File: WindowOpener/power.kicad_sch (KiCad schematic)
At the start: 18 parts, among them J10 Batt_Conn1, J11 Batt_Conn2, J12 Batt_Conn2, J3 Batt_Conn1, J4 Batt_Conn2, J5 Batt_Conn1, J6 Batt_Conn2, J7 Batt_Conn1, J8 Batt_Conn2, J9 Batt_Conn2, U3 AZ1117CH2-3.3, U4 PAM2421AECADJR

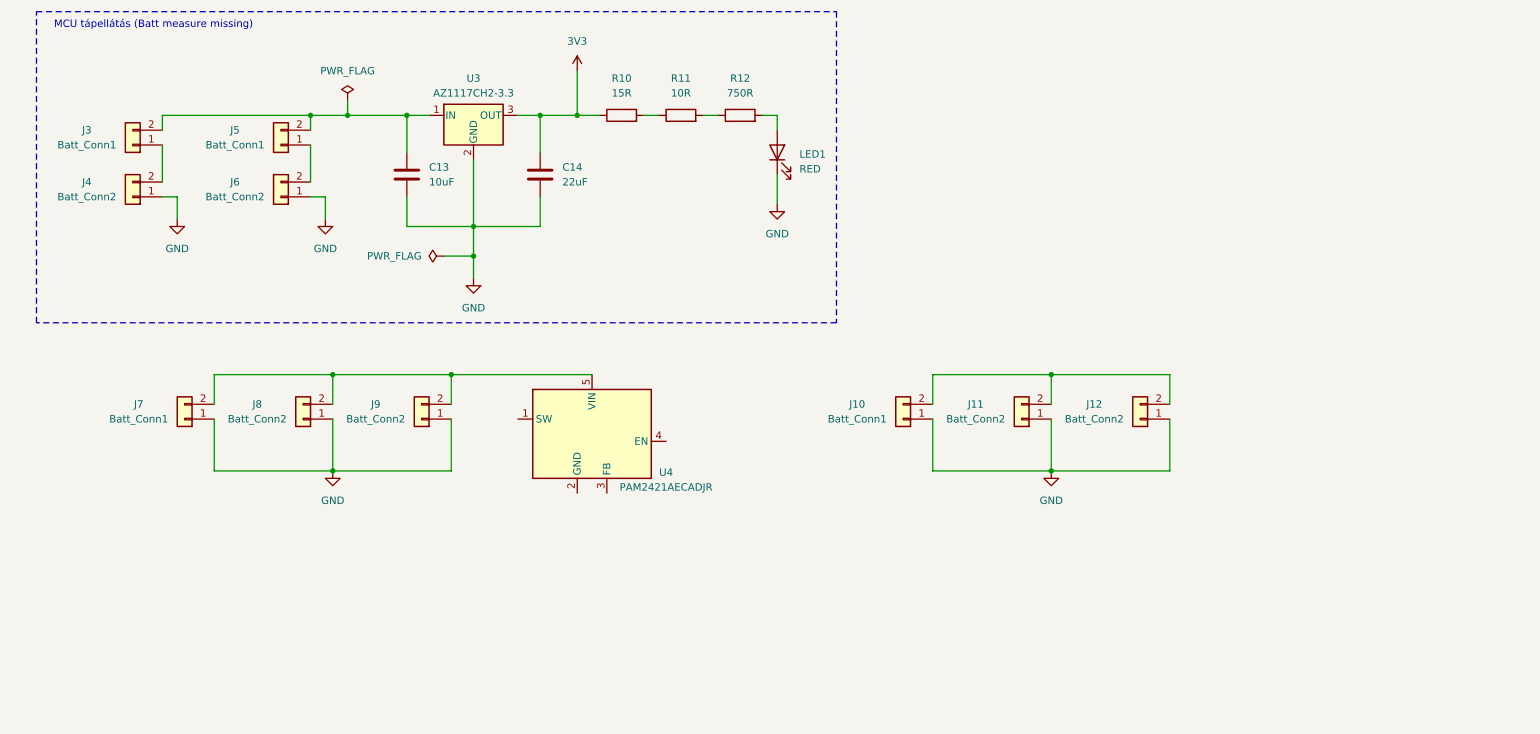
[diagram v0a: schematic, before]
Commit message: v0.2
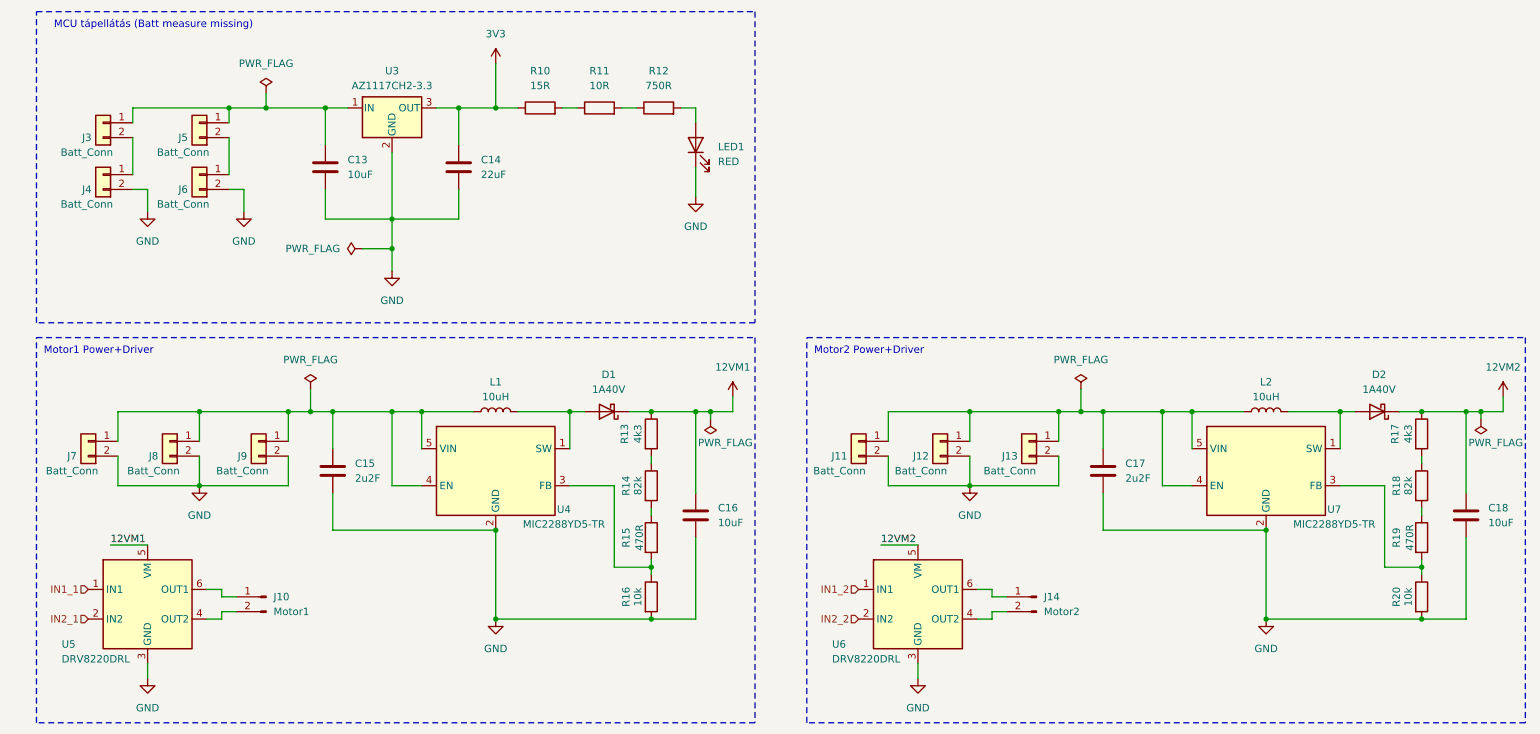
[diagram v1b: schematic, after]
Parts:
- removed J10: Batt_Conn1, Battery:BatteryHolder_Keystone_1042_1x18650, symbol Connector_Generic:Conn_01x02
- added C15, C17: 2u2F, Capacitor_SMD:C_1206_3216Metric_Pad1.33x1.80mm_HandSolder, symbol Device:C
- added C16, C18: 10uF, Capacitor_SMD:C_1206_3216Metric_Pad1.33x1.80mm_HandSolder, symbol Device:C
- added D1, D2: 1A40V, SmartHomeFootprints:1N5819HW-7-F, symbol Device:D_Schottky
- added J10: Motor1, Connector_PinHeader_2.54mm:PinHeader_1x02_P2.54mm_Vertical, symbol Connector:Conn_01x02_Pin
- added J13: Batt_Conn, Battery:BatteryHolder_Keystone_1042_1x18650, symbol Connector_Generic:Conn_01x02
- added J14: Motor2, Connector_PinHeader_2.54mm:PinHeader_1x02_P2.54mm_Vertical, symbol Connector:Conn_01x02_Pin
- added L1, L2: 10uH, Inductor_SMD:L_1210_3225Metric_Pad1.42x2.65mm_HandSolder, symbol Device:L
- added R13, R17: 4k3, Resistor_SMD:R_1206_3216Metric_Pad1.30x1.75mm_HandSolder, symbol Device:R
- added R14, R18: 82k, Resistor_SMD:R_1206_3216Metric_Pad1.30x1.75mm_HandSolder, symbol Device:R
- added R15, R19: 470R, Resistor_SMD:R_1206_3216Metric_Pad1.30x1.75mm_HandSolder, symbol Device:R
- added R16, R20: 10k, Resistor_SMD:R_2010_5025Metric_Pad1.40x2.65mm_HandSolder, symbol Device:R
- added U5, U6: DRV8220DRL, Package_TO_SOT_SMD:SOT-563, symbol Driver_Motor:DRV8220DRL
- added U7: MIC2288YD5-TR, Package_TO_SOT_SMD:TSOT-23-5_HandSoldering, symbol SmartHomeSymbols:PAM2421AECADJR
- C13: footprint Capacitor_SMD:C_2220_5750Metric_Pad1.97x5.40mm_HandSolder -> Capacitor_SMD:C_1206_3216Metric_Pad1.33x1.80mm_HandSolder; Store link https://hu.farnell.com/chemi-con/kts500b106m55n0t00/cap-mlc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 -> https://hu.farnell.com/multicomp-pro/1206x106k160ct/cap-10-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
- J11, J12, J4, J6, J8, J9: value Batt_Conn2 -> Batt_Conn
- J3, J5, J7: value Batt_Conn1 -> Batt_Conn
- R11, R12: footprint LED_SMD:LED_1206_3216Metric_Pad1.42x1.75mm_HandSolder -> Resistor_SMD:R_1206_3216Metric_Pad1.30x1.75mm_HandSolder
- U4: value PAM2421AECADJR -> MIC2288YD5-TR; footprint (none) -> Package_TO_SOT_SMD:TSOT-23-5_HandSoldering; Store link (none) -> https://hu.farnell.com/microchip/mic2288yd5-tr/switching-re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
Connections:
- net GND: now also J11.2 (Pin_1), J12.2 (Pin_1), J4.2 (Pin_1), J6.2 (Pin_1), J7.2 (Pin_1), J8.2 (Pin_1), J9.2 (Pin_1), U4.2 (GND), C15.2, C16.2, C17.2, C18.2, J13.2 (Pin_1), R16.2, R20.2, U5.3 (GND), U6.3 (GND), U7.2 (GND); no longer J11.1 (Pin_1), J12.1 (Pin_1), J4.1 (Pin_1), J6.1 (Pin_1), J7.1 (Pin_1), J8.1 (Pin_1), J9.1 (Pin_1)
- net at J3.1 (Pin_2): now also C13.1, J5.1 (Pin_2), U3.1 (IN); no longer J4.2 (Pin_2)
- net at U4.1 (SW): now also D1.2 (A), L1.2
- net at U4.3 (FB): now also R15.2, R16.1
- net at U4.4 (EN): now also J7.1 (Pin_2), J8.1 (Pin_2), J9.1 (Pin_2), U4.5 (VIN), C15.1, L1.1
- new net: D2.2 (A), L2.2, U7.1 (SW)
- new net: J5.2 (Pin_1), J6.1 (Pin_2)
- new net: R13.2, R14.1
- new net: R17.2, R18.1
- new net: C17.1, J11.1 (Pin_2), J12.1 (Pin_2), J13.1 (Pin_2), L2.1, U7.4 (EN), U7.5 (VIN)
- new net: J10.1 (Pin_2), U5.6 (OUT1)
- new net: J10.2 (Pin_1), U5.4 (OUT2)
- new net: J14.1 (Pin_2), U6.6 (OUT1)
- new net: J14.2 (Pin_1), U6.4 (OUT2)
- new net: R18.2, R19.1
- new net: R19.2, R20.1, U7.3 (FB)
- new net: J3.2 (Pin_1), J4.1 (Pin_2)
- new net: R14.2, R15.1
- new net 12VM1: C16.1, D1.1 (K), R13.1, U5.5 (VM)
- new net 12VM2: C18.1, D2.1 (K), R17.1, U6.5 (VM)
- new net IN1_1: U5.1 (IN1)
- new net IN1_2: U6.1 (IN1)
- new net IN2_1: U5.2 (IN2)
- new net IN2_2: U6.2 (IN2)
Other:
- note added: "Motor1 Power+Driver"
- note added: "Motor2 Power+Driver"
- moved on the sheet: C13, C14, J3, LED1, R10, R11, R12, U3, U4
